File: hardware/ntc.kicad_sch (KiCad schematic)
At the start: 3 parts

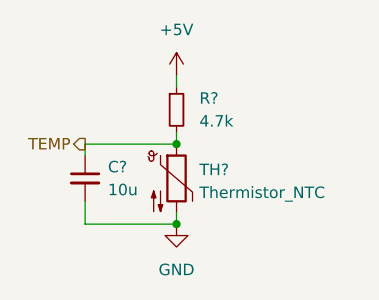
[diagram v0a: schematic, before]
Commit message: Annotate schematic
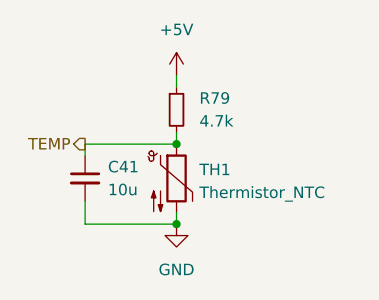
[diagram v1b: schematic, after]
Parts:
- gave numbers to parts that had none: 3
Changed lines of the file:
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@@
   (symbol (lib_id "Device:C_Small") (at 138.43 102.87 0) (unit 1)
     (in_bom yes) (on_board yes) (fields_autoplaced)
-    (property "Reference" "C?" (id 0) (at 140.97 101.6062 0)
+    (property "Reference" "C41" (id 0) (at 140.97 101.6062 0)
       (effects (font (size 1.27 1.27)) (justify left))
     )
@@
   (symbol (lib_id "power:GND") (at 148.59 107.95 0) (unit 1)
     (in_bom yes) (on_board yes) (fields_autoplaced)
-    (property "Reference" "#PWR?" (id 0) (at 148.59 114.3 0)
+    (property "Reference" "#PWR044" (id 0) (at 148.59 114.3 0)
       (effects (font (size 1.27 1.27)) hide)
     )
@@
   (symbol (lib_id "Device:R_Small") (at 148.59 95.25 0) (unit 1)
     (in_bom yes) (on_board yes) (fields_autoplaced)
-    (property "Reference" "R?" (id 0) (at 151.13 93.9799 0)
+    (property "Reference" "R79" (id 0) (at 151.13 93.9799 0)
       (effects (font (size 1.27 1.27)) (justify left))
     )
@@
   (symbol (lib_id "Device:Thermistor_NTC") (at 148.59 102.87 0) (unit 1)
     (in_bom yes) (on_board yes) (fields_autoplaced)
-    (property "Reference" "TH?" (id 0) (at 151.13 101.9174 0)
+    (property "Reference" "TH1" (id 0) (at 151.13 101.9174 0)
       (effects (font (size 1.27 1.27)) (justify left))
     )
@@
   (symbol (lib_id "power:+5V") (at 148.59 91.44 0) (unit 1)
     (in_bom yes) (on_board yes) (fields_autoplaced)
-    (property "Reference" "#PWR?" (id 0) (at 148.59 95.25 0)
+    (property "Reference" "#PWR043" (id 0) (at 148.59 95.25 0)
       (effects (font (size 1.27 1.27)) hide)
     )

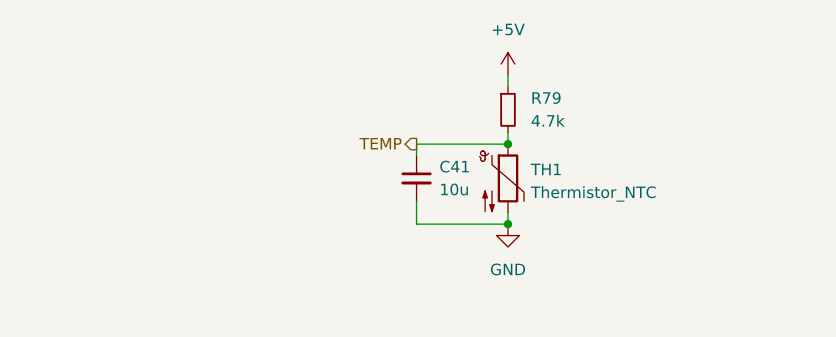
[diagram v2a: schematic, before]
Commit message: Thermistors filtering
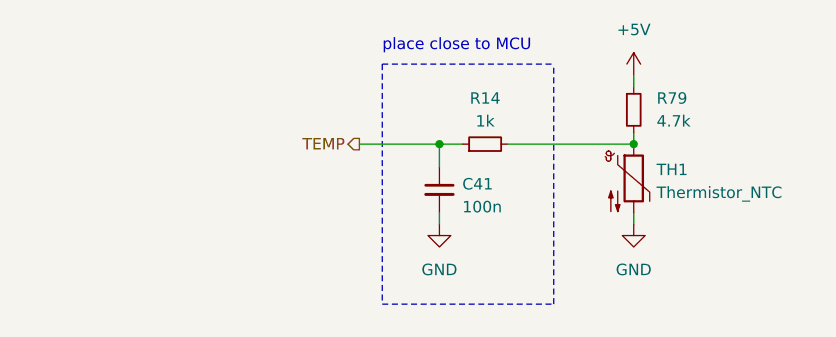
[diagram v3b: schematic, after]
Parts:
- added R14: 1k, symbol Device:R_Small
- C41: value 10u -> 100n
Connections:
- net TEMP: now also R14.1; no longer R79.2, TH1.1
- new net: R14.2, R79.2, TH1.1
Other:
- note added: "place close to MCU"
- moved on the sheet: R79, TH1

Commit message: Work on thermal
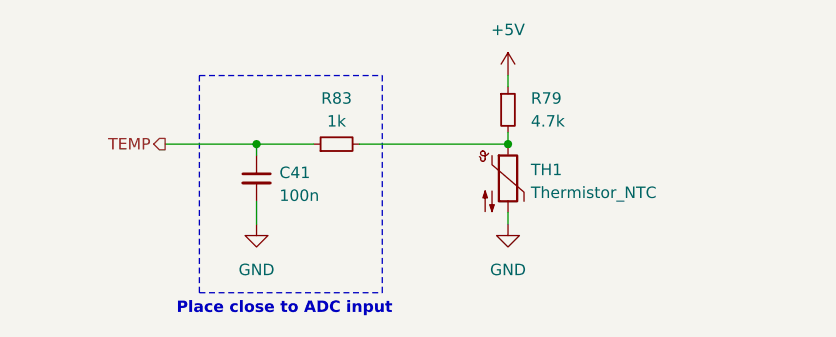
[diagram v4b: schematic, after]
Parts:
- removed R14: 1k, symbol Device:R_Small
- added R83: 1k, symbol Device:R_Small
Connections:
- net TEMP: now also R83.1
- net at R79.2, TH1.1: now also R83.2
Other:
- note added: "Place close to ADC input"
- note removed: "place close to MCU"
- moved on the sheet: R79, TH1

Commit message: Charger enable circiut and more ext NTC
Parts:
- TH1: footprint (none) -> Resistor_SMD:R_2010_5025Metric
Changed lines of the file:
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@@
           (reference "C43") (unit 1)
         )
+        (path "/3e668e3e-3e16-4665-a807-4735962c41d3/95476253-acbc-4b80-80be-f4a25f0f1538/8331fb18-4942-4880-a12f-c73df369bf91"
+          (reference "C52") (unit 1)
+        )
+        (path "/3e668e3e-3e16-4665-a807-4735962c41d3/95476253-acbc-4b80-80be-f4a25f0f1538/17178c98-8beb-40cf-b2d2-307d0f34da43"
+          (reference "C53") (unit 1)
+        )
       )
     )
@@
           (reference "#PWR048") (unit 1)
         )
+        (path "/3e668e3e-3e16-4665-a807-4735962c41d3/95476253-acbc-4b80-80be-f4a25f0f1538/8331fb18-4942-4880-a12f-c73df369bf91"
+          (reference "#PWR078") (unit 1)
+        )
+        (path "/3e668e3e-3e16-4665-a807-4735962c41d3/95476253-acbc-4b80-80be-f4a25f0f1538/17178c98-8beb-40cf-b2d2-307d0f34da43"
+          (reference "#PWR081") (unit 1)
+        )
       )
     )
@@
           (reference "R81") (unit 1)
         )
+        (path "/3e668e3e-3e16-4665-a807-4735962c41d3/95476253-acbc-4b80-80be-f4a25f0f1538/8331fb18-4942-4880-a12f-c73df369bf91"
+          (reference "R97") (unit 1)
+        )
+        (path "/3e668e3e-3e16-4665-a807-4735962c41d3/95476253-acbc-4b80-80be-f4a25f0f1538/17178c98-8beb-40cf-b2d2-307d0f34da43"
+          (reference "R99") (unit 1)
+        )
       )
     )
@@
       (effects (font (size 1.27 1.27)) (justify left))
     )
-    (property "Footprint" "" (at 148.59 101.6 0)
+    (property "Footprint" "Resistor_SMD:R_2010_5025Metric" (at 148.59 101.6 0)
       (effects (font (size 1.27 1.27)) hide)
     )
@@
           (reference "TH3") (unit 1)
         )
+        (path "/3e668e3e-3e16-4665-a807-4735962c41d3/95476253-acbc-4b80-80be-f4a25f0f1538/8331fb18-4942-4880-a12f-c73df369bf91"
+          (reference "TH5") (unit 1)
+        )
+        (path "/3e668e3e-3e16-4665-a807-4735962c41d3/95476253-acbc-4b80-80be-f4a25f0f1538/17178c98-8beb-40cf-b2d2-307d0f34da43"
+          (reference "TH6") (unit 1)
+        )
       )
     )
@@
           (reference "#PWR057") (unit 1)
         )
+        (path "/3e668e3e-3e16-4665-a807-4735962c41d3/95476253-acbc-4b80-80be-f4a25f0f1538/8331fb18-4942-4880-a12f-c73df369bf91"
+          (reference "#PWR076") (unit 1)
+        )
+        (path "/3e668e3e-3e16-4665-a807-4735962c41d3/95476253-acbc-4b80-80be-f4a25f0f1538/17178c98-8beb-40cf-b2d2-307d0f34da43"
+          (reference "#PWR079") (unit 1)
+        )
       )
     )
@@
           (reference "R84") (unit 1)
         )
+        (path "/3e668e3e-3e16-4665-a807-4735962c41d3/95476253-acbc-4b80-80be-f4a25f0f1538/8331fb18-4942-4880-a12f-c73df369bf91"
+          (reference "R96") (unit 1)
+        )
+        (path "/3e668e3e-3e16-4665-a807-4735962c41d3/95476253-acbc-4b80-80be-f4a25f0f1538/17178c98-8beb-40cf-b2d2-307d0f34da43"
+          (reference "R98") (unit 1)
+        )
       )
     )
@@
           (reference "#PWR047") (unit 1)
         )
-      )
+        (path "/3e668e3e-3e16-4665-a807-4735962c41d3/95476253-acbc-4b80-80be-f4a25f0f1538/8331fb18-4942-4880-a12f-c73df369bf91"
+          (reference "#PWR077") (unit 1)
+        )
+        (path "/3e668e3e-3e16-4665-a807-4735962c41d3/95476253-acbc-4b80-80be-f4a25f0f1538/17178c98-8beb-40cf-b2d2-307d0f34da43"
+          (reference "#PWR080") (unit 1)
+        )
+      )

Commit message: OLED screen
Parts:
- TH1: footprint Resistor_SMD:R_2010_5025Metric -> Connector_JST:JST_XH_B2B-XH-A_1x02_P2.50mm_Vertical
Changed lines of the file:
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@@
       (effects (font (size 1.27 1.27)) (justify left))
     )
-    (property "Footprint" "Resistor_SMD:R_2010_5025Metric" (at 148.59 101.6 0)
+    (property "Footprint" "Connector_JST:JST_XH_B2B-XH-A_1x02_P2.50mm_Vertical" (at 148.59 101.6 0)
       (effects (font (size 1.27 1.27)) hide)
     )

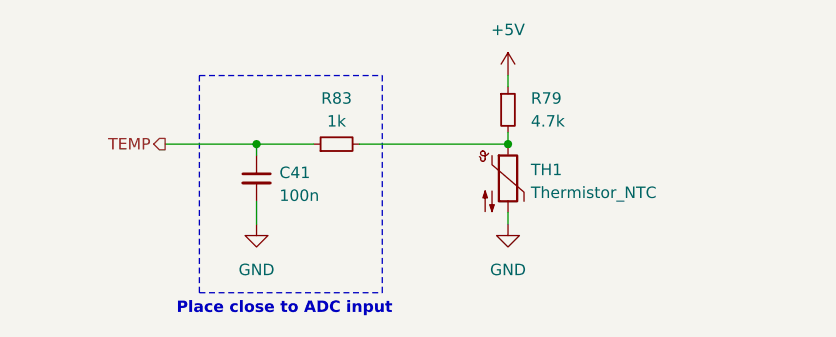
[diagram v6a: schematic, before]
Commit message: Charge monitor complete
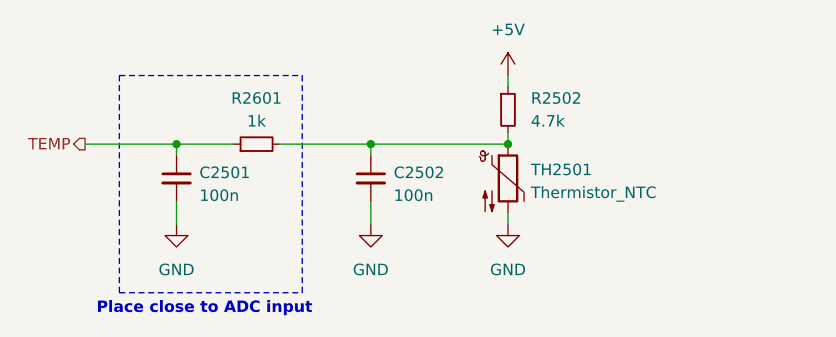
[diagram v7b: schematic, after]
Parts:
- added C2502: 100n, symbol Device:C_Small
- renumbered C41 to C2501, R79 to R2502, R83 to R2601, TH1 to TH2501
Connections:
- net GND: now also C2502.2
- net at R2502.2, R2601.2, TH2501.1: now also C2502.1
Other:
- moved on the sheet: C2501, R2601
